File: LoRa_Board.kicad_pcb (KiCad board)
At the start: 4 copper layers, 100 x 54 mm, 121 parts, among them IC2 RF_Switch_PE42440MLBB-Z, J10 SMA PCB END LAUNCH JACK ROUND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, J11 Coin Battery Jumper, J2 UART1_HDR, J3 SWDB, J4 USB_C_Receptacle_USB2.0_16P, J5 I/O_HDR, J6 BOOT0_Jumper, J7 I2C2_Headers, J8 PWR_SRC_JMP, J9 I2C1_Headers, Q2 MOSFET_SI2333DDS-T1-BE3, SW2 Switch_NX3L1T3157GM,115, SW3 Switch_NX3L1T3157GM,115, U1 USBLC6-2SC6, U3 SN74LVC1G07DBVR, U4 STM32WL55CCU6, U6 FT230XS

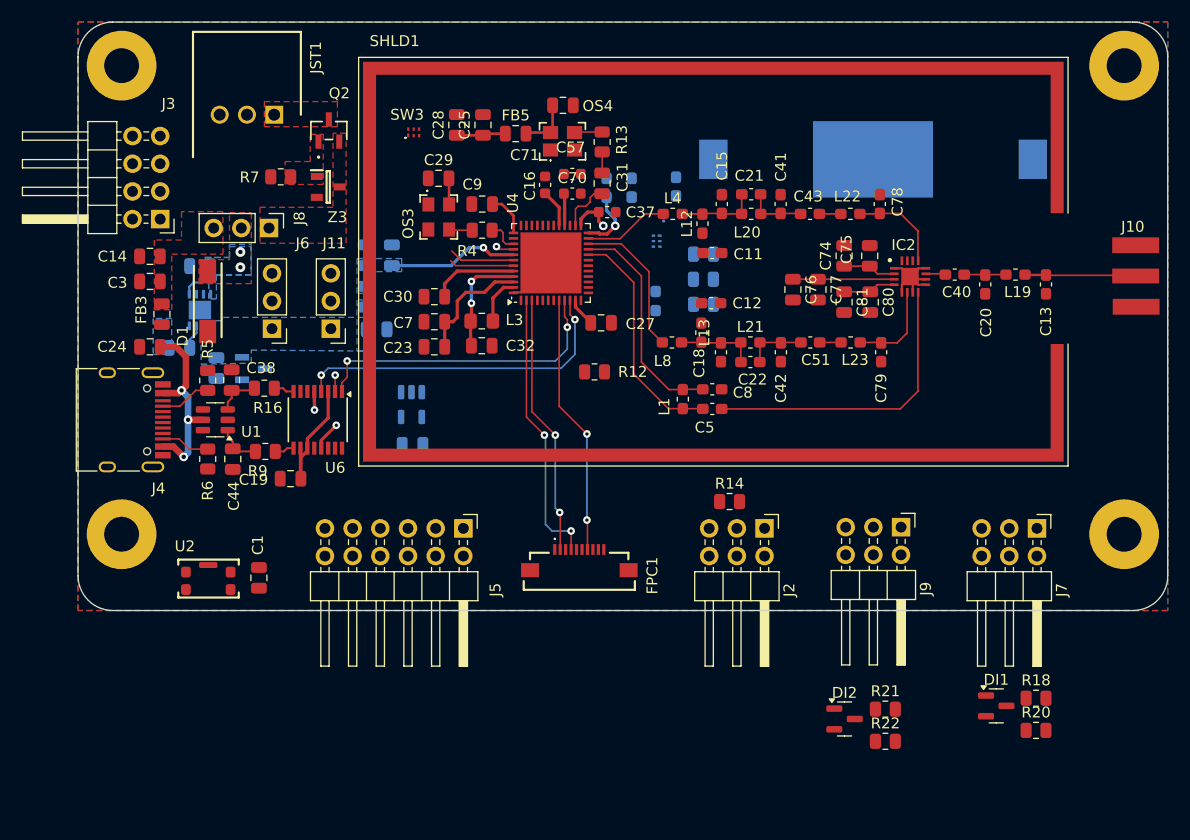
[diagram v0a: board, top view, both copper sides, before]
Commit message: Update
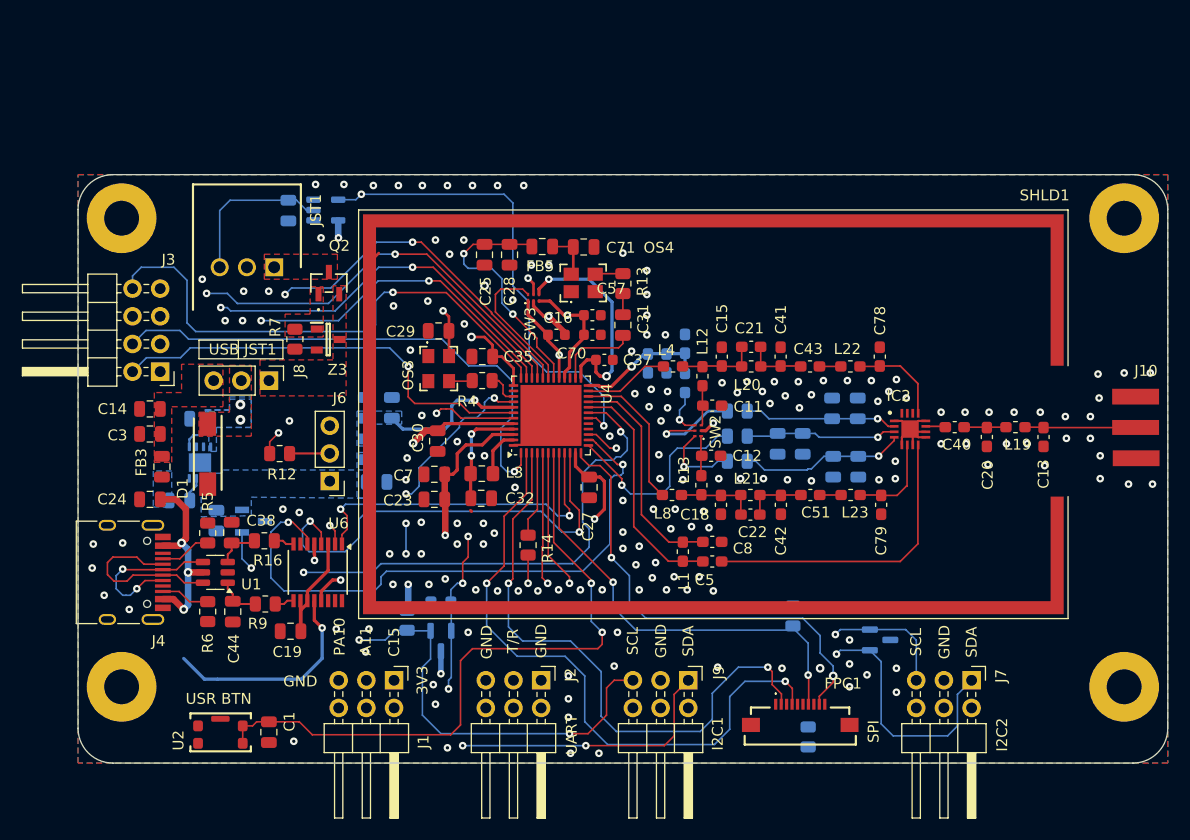
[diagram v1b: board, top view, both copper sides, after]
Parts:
- removed BH2: Battery_Holder_1060TR, Personal_Project:Battery_Holder_1060TR
- removed C9: 100n, Capacitor_SMD:C_0805_2012Metric
- removed J11: Coin Battery Jumper, Connector_PinHeader_2.54mm:PinHeader_1x03_P2.54mm_Vertical
- removed J5: I/O_HDR, Connector_PinHeader_2.54mm:PinHeader_2x06_P2.54mm_Horizontal
- added C35: 100n, Capacitor_SMD:C_0805_2012Metric, F.Cu at (138.1, 84.7)
- added G***: LOGO, Personal_Project:PCB_Logo, B.Cu at (186.4, 78.2)
- added J1: I/O_HDR, Connector_PinHeader_2.54mm:PinHeader_2x03_P2.54mm_Horizontal, F.Cu at (130.0, 114.4)
- C25: value 100n_CL21B104KCFNNNE -> 100n_CC0402KRX7R7BB104
- C28: value 47p_KGQ21HCG2D470JT -> 47p_CC0402JRNPO9BN470
- C71: value 10n -> 220n
- C74, C75, C76, C77, C80, C81, DI1, DI2, R18, R20, R21, R22: moved to B.Cu
- SW2: moved to F.Cu
- moved R22 45.3 mm to (131.2, 108.9), turned to -90 degrees
- moved R21 41.9 mm to (134.3, 107.4)
- moved DI2 37.7 mm to (134.3, 110.8), turned to -90 degrees
- moved R12 29.9 mm to (119.5, 93.6), turned to 180 degrees
- moved J2 24.8 mm to (143.5, 114.4)
- moved FPC1 24.8 mm to (167.3, 118.2)
- moved R20 24.7 mm to (166.6, 108.5), turned to 90 degrees
- moved C34 24.3 mm to (120.3, 71.3), turned to -90 degrees
- moved J9 24.1 mm to (157.0, 114.4)
- moved R18 21.2 mm to (168.0, 119.6), turned to 90 degrees
- moved U3 19.5 mm to (123.7, 71.2), turned to 0 degrees
- moved R14 18.9 mm to (142.3, 102.0), turned to -90 degrees
- moved SW3 18.7 mm to (142.8, 79.3)
- moved SW2 17.8 mm to (157.9, 91.5), turned to 90 degrees
- moved C4 17.0 mm to (155.0, 85.3), turned to -90 degrees
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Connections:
- net /Interfaces/I/O_HDR4 renamed /STM32WL55CCU6/PB2_RFVCTRL
- C11 pad 2: /Antenna/Y1 -> /Antenna/Y0
- C12 pad 2: /Antenna/Y0 -> /Antenna/Y1
- L12 pad 1: /Antenna/Y1 -> /Antenna/Y0
- L13 pad 2: /Antenna/Y0 -> /Antenna/Y1
- U4 pad 16: /Interfaces/I/O_HDR1 -> /STM32WL55CCU6/PA8_MCO
- U4 pad 17: /Interfaces/USR_BTN -> /STM32WL55CCU6/PA9_USR_BTN
- U4 pad 33: /Interfaces/I/O_HDR0 -> /Interfaces/I/O_HDR2
- U4 pad 34: /Interfaces/I/O_HDR2 -> /Interfaces/I/O_HDR1
- U4 pad 37: VBAT+ -> +3.3V
- U4 pad 40: /Interfaces/I/O_HDR5 -> /Interfaces/I/O_HDR0
- U4 pad 7: /Interfaces/I/O_HDR3 -> /Interfaces/USR_BTN
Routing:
- net +3.3V: track 27.6 -> 180.1 mm, vias 0 -> 10
- net /Interfaces/NRST: track 0.00 -> 117.8 mm, vias 0 -> 3
- net /Interfaces/I2C1_SCL_HDR: track 0.00 -> 112.3 mm, vias 0 -> 4
- net /Interfaces/I/O_HDR2: track 0.00 -> 87.2 mm, vias 0 -> 2
- net /Interfaces/I/O_HDR1: track 0.00 -> 84.3 mm, vias 0 -> 2
- net /Interfaces/I2C2_SDA_HDR: track 0.00 -> 66.8 mm, vias 0 -> 2
- net /STM32WL55CCU6/BOOT0: track 0.00 -> 63.3 mm, vias 0 -> 3
- net /Interfaces/USR_BTN: track 0.00 -> 61.5 mm, vias 0 -> 2
- net /Interfaces/I2C1_SDA_HDR: track 5.95 -> 66.3 mm, vias 0 -> 6
- net /STM32WL55CCU6/PB12_LPUART1_RTS: track 1.51 -> 57.9 mm, vias 1 -> 3
- net /STM32WL55CCU6/PA6_LPUART1_CTS: track 0.00 -> 55.2 mm, vias 0 -> 2
- net /Interfaces/I2C2_SCL_HDR: track 0.00 -> 53.7 mm, vias 0 -> 2
- net /Interfaces/SWO: track 0.00 -> 48.9 mm, vias 0 -> 1
- net /Interfaces/SWDIO: track 0.00 -> 48.5 mm, vias 0 -> 1
- net /Interfaces/SPI_CS: track 0.00 -> 42.4 mm, vias 0 -> 2
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- added copper zone on In2.Cu, net +3.3V
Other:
- board text added: "3V3"
- board text added: "A11"
- board text added: "C15"
- board text added: "GND"
- board text added: "I2C1"
- board text added: "I2C2"
- board text added: "LORA BOARD Revision: REV B Designer: Peter Hancak MCU: STM32WL55CCU6 LDO: LDLN050PU33R VIN: 2.7 to 6.5V"
- board text added: "PA10"
- board text added: "SCL"
- board text added: "SD NR SO SC"
- board text added: "SDA"
- board text added: "SPI"
- board text added: "T/R"
- board text added: "UART"
- board text added: "USB JST1"
- board text added: "USR BTN"
